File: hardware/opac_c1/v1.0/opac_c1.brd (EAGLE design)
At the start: 49 x 90.9 mm, 63 parts, among them IC1 DS3231WIDE, IC2 CP2102, IC3 ATSHA204_SOIC8, IC4 MP1584, SW1 RESET

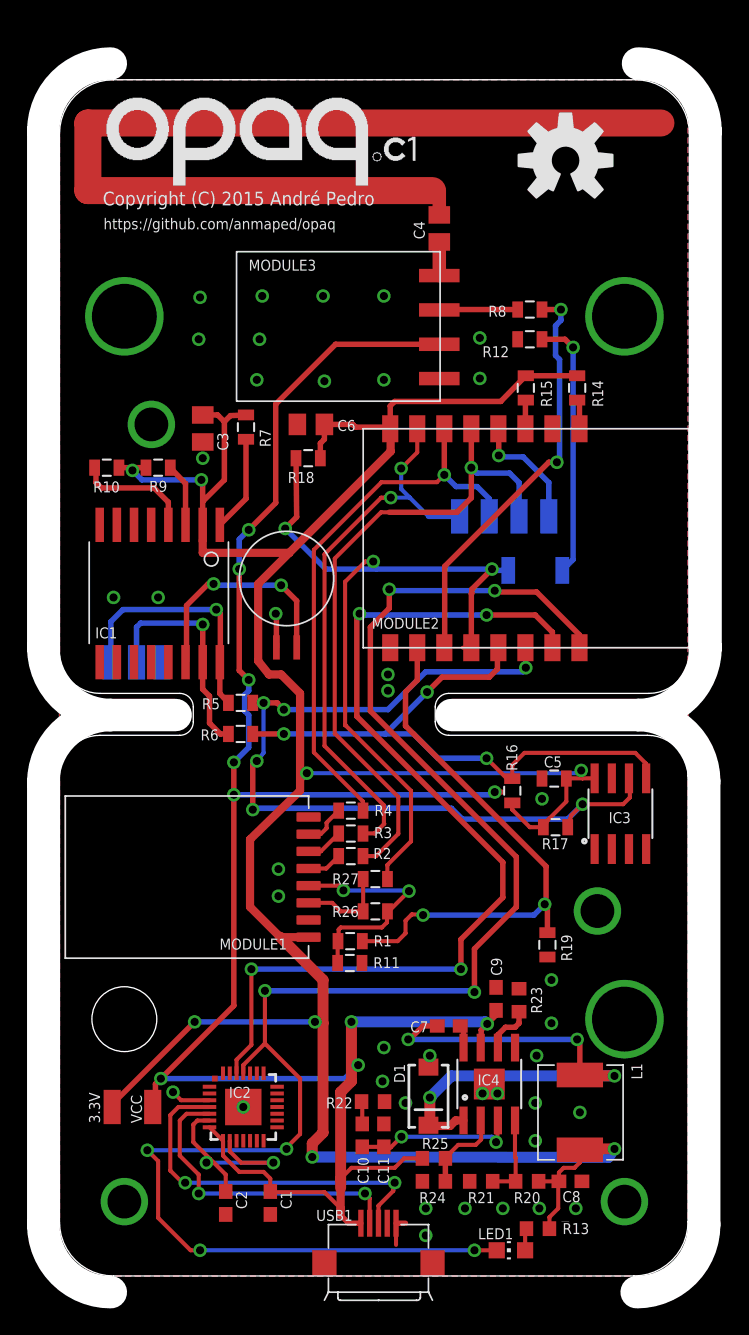
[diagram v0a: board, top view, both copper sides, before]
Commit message: Opaq.c1 revision 2.
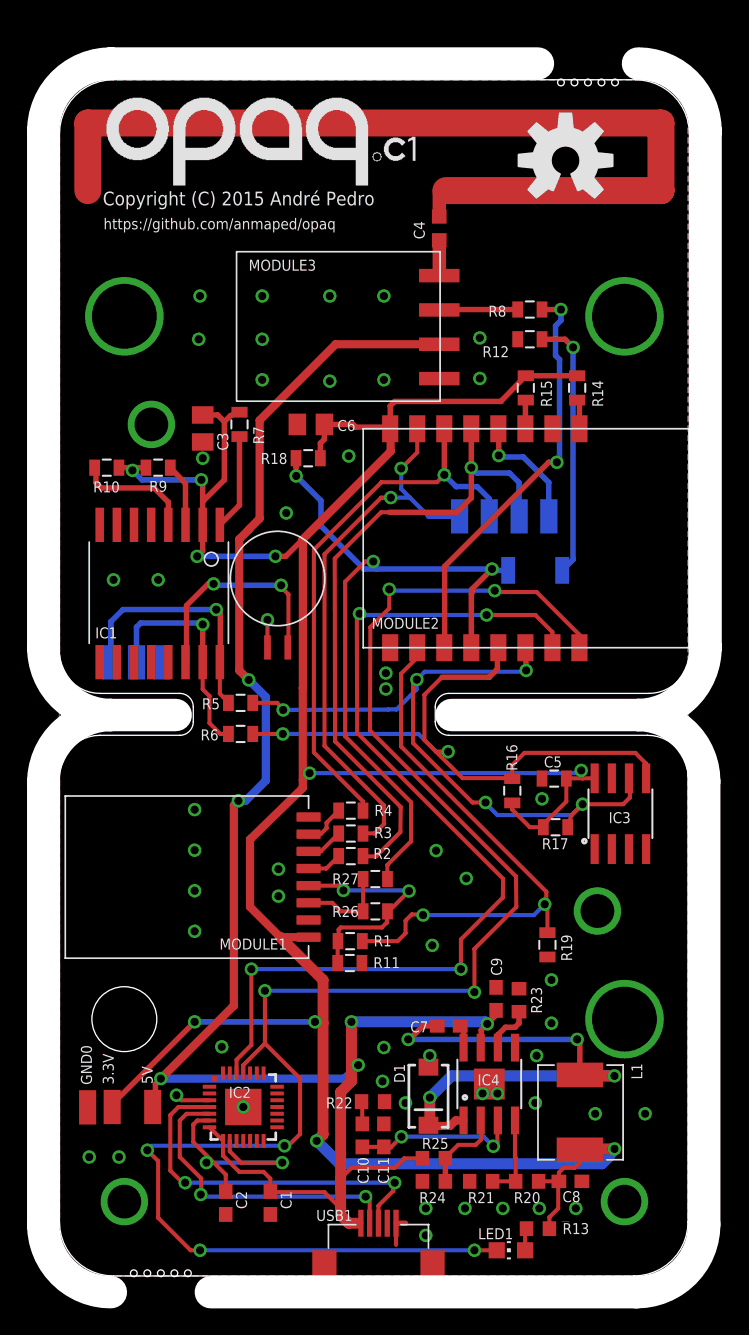
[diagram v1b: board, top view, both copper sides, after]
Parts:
- added GND0: (no value), wirepad:SMD1,27-2,54
- C4: device resistor:C0805K -> resistor:C0603K
- moved U$3 0.66 mm to (16.1, 50.1)
- moved R7 0.52 mm to (13.3, 61.5)
- renumbered VCC to 5V
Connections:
- net GND: now also GND0.1
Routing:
- net N$22: track 72.9 -> 0.00 mm
- net N$29: track 0.00 -> 68.3 mm
- net VCC: track 156.7 -> 138.0 mm, vias 10 -> 6
- net SCL_C: track 63.9 -> 51.3 mm, vias 6 -> 5
- net CE_NRF24: track 58.6 -> 55.6 mm
- net 3.3V: track 204.1 -> 201.3 mm, vias 8 -> 10
- net SDA_C: track 45.6 -> 47.8 mm, vias 3 -> 2
- net RST: track 17.0 -> 18.3 mm
- net GND: track 7.65 -> 7.17 mm, vias 40 -> 52
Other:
- outline, holes or cut-outs redrawn
- board text added: "Released under the Creative Commons Attribution Share-Alike 4.0 License"
- board text removed: "André M. Pedro"

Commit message: Opaq C1 hardware revision 3.
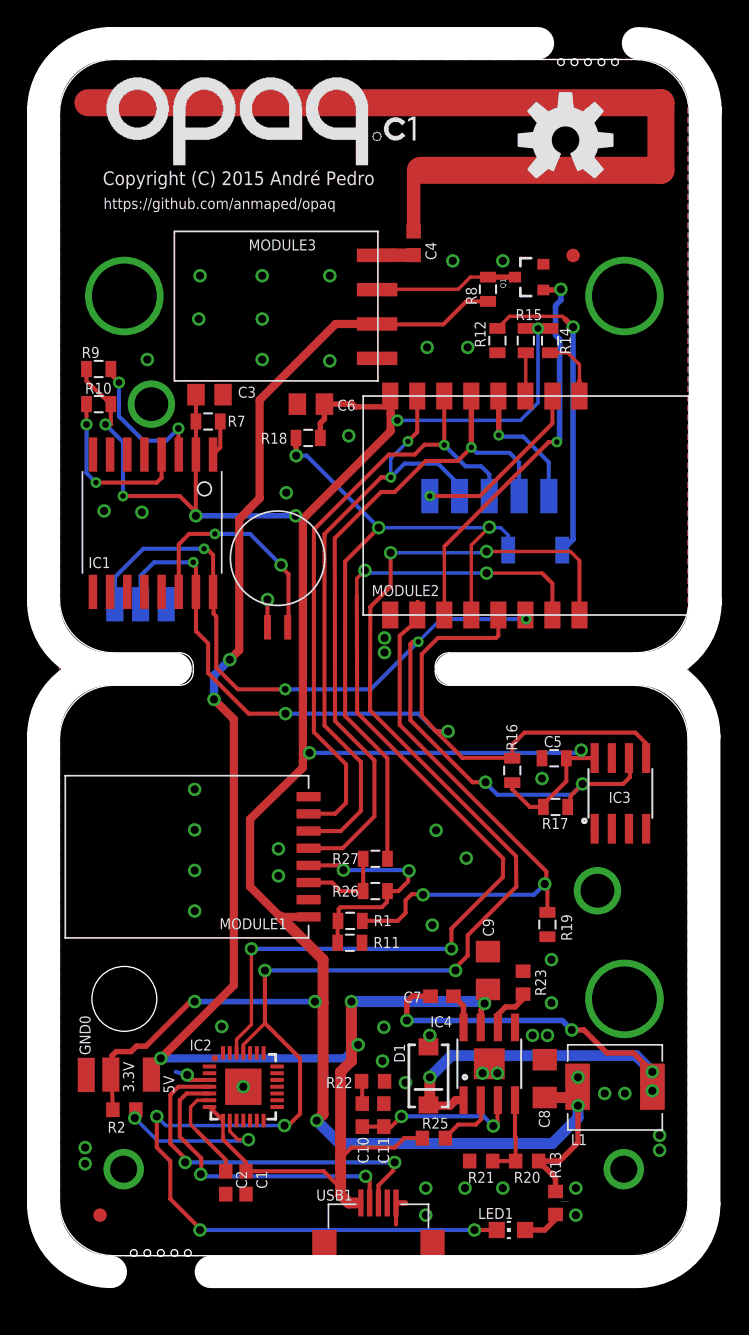
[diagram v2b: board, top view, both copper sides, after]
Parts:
- removed CE: (no value), wirepad:SMD1,27-2,54
- removed R24: (no value), resistor:R0603
- removed R3, R4, R5, R6: (no value), resistor:0805
- added ADC, GPIO16: (no value), wirepad:SMD1,27-2,54
- added JP2, JP3: FIDUCIAL1X2.5, SparkFun:FIDUCIAL-1X2.5
- added Q1: MMBT2222A, SparkFun-DiscreteSemi:SOT23-3
- C8, C9: device resistor:C0603 -> resistor:C3216
- R2: device resistor:0805 -> resistor:R0603
- SW1: value RESET -> PROG
- moved R2 25.2 mm to (4.80, 10.8), turned to 0 degrees
- moved R9 8.52 mm to (2.90, 65.6)
- moved C8 7.83 mm to (35.9, 13.1), turned to 90 degrees
- moved IC1 5.22 mm to (12.0, 58.0)
- moved JP1 4.84 mm to (18.5, 70.2)
- moved R10 4.74 mm to (2.90, 63.0)
- moved GND 4.31 mm to (7.90, 48.2)
- moved SCL 4.31 mm to (4.10, 48.2)
- moved SDA 4.31 mm to (6.00, 48.2)
- moved R14 4.03 mm to (36.3, 67.7)
- moved R15 3.50 mm to (34.5, 67.7)
- moved R8 3.44 mm to (31.7, 71.5), turned to 90 degrees
- moved L1 3.22 mm to (41.1, 12.5), turned to 180 degrees
- moved C3 2.55 mm to (11.1, 63.7), turned to 0 degrees
- moved MODULE2 2.42 mm to (22.5, 63.6)
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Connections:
- removed net N$5: MODULE1.6, R3.2
- removed net N$6: MODULE1.7, R4.2
- removed net SCL_C_A: IC1.16, R5.1, SCL.1
- removed net SDA_C_A: IC1.15, R6.1, SDA.1
- new net ADC_IN: ADC.1, MODULE2.10
- net 3.3V: now also R2.1
- net CE_EXTRA: now also GPIO16.1; no longer CE.1
- net GND: now also Q1.2; no longer R24.1
- net MISO_NRF24: now also MODULE1.7; no longer R4.1
- net MOSI_NRF24: now also MODULE1.6; no longer R3.1
- net N$19: now also Q1.3
- net N$32: no longer R24.2
- net N$4: now also C2.1, IC2.6; no longer MODULE1.5, R2.2
- net RST: now also R2.2; no longer C2.1, IC2.6
- net SCK_NRF24: now also MODULE1.5; no longer R2.1
- net SCL_C: now also IC1.16, SCL.1; no longer R5.2
- net SDA_C: now also IC1.15, SDA.1; no longer R6.2
- net SIGNAL433: now also Q1.1; no longer R8.1
- net VCC: now also R8.1
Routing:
- net SDA_C: track 47.8 -> 70.1 mm, vias 2 -> 3
- net SCL_C: track 51.3 -> 73.4 mm, vias 5 -> 6
- net SCL_C_A: track 18.8 -> 0.00 mm, vias 1 -> 0
- net SDA_C_A: track 17.0 -> 0.00 mm, vias 1 -> 0
- net ADC_IN: track 0.00 -> 13.3 mm, vias 0 -> 1
- net 3.3V: track 201.3 -> 214.1 mm, vias 10 -> 13
- net N$17: track 39.8 -> 47.2 mm, vias 4 -> 5
- net RST: track 18.3 -> 11.5 mm
- net N$2: track 4.68 -> 11.2 mm, vias 0 -> 2
- net N$4: track 2.61 -> 7.58 mm
- net N$19: track 5.81 -> 10.6 mm
- net MOSI_NRF24: track 42.3 -> 47.0 mm
- net MISO_NRF24: track 41.5 -> 46.0 mm
- net N$10: track 7.13 -> 2.67 mm
- net N$24: track 8.79 -> 12.8 mm, vias 0 -> 2
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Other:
- outline, holes or cut-outs redrawn
